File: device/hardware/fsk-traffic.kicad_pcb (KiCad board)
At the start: 2 copper layers, 79 x 41.5 mm, 43 parts, among them J1 JTAG, J2 USB_C, J3 2EDGV-5.08-03P, J4 2EDGV-5.08-03P, J5 2EDGV-5.08-03P, Q1 MMBT5551, Q2 AO3401A, Q3 MMBT5551, Q4 AO3401A, U1 XC6206P332MR, U2 MT3608, U3 STM32F070F6Px, Y1 12MHz

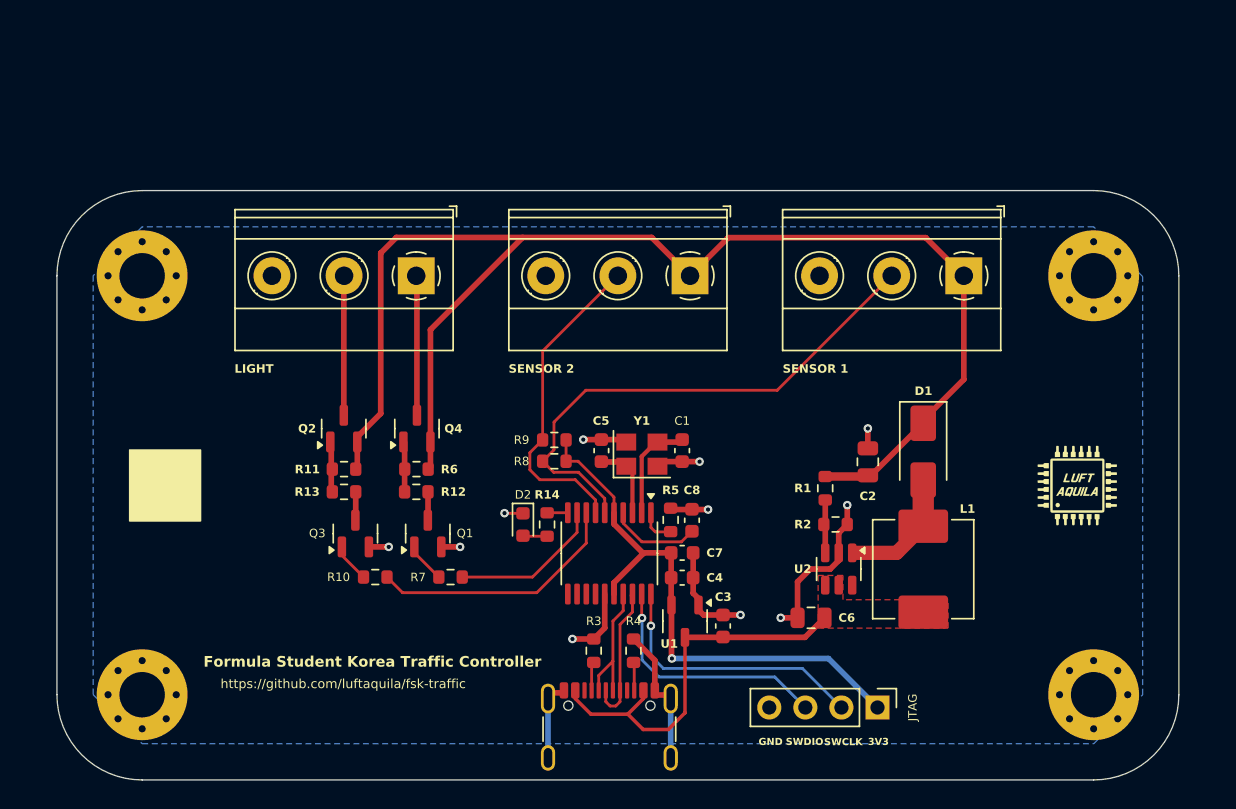
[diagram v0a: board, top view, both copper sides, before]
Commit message: fix: isolation & filter
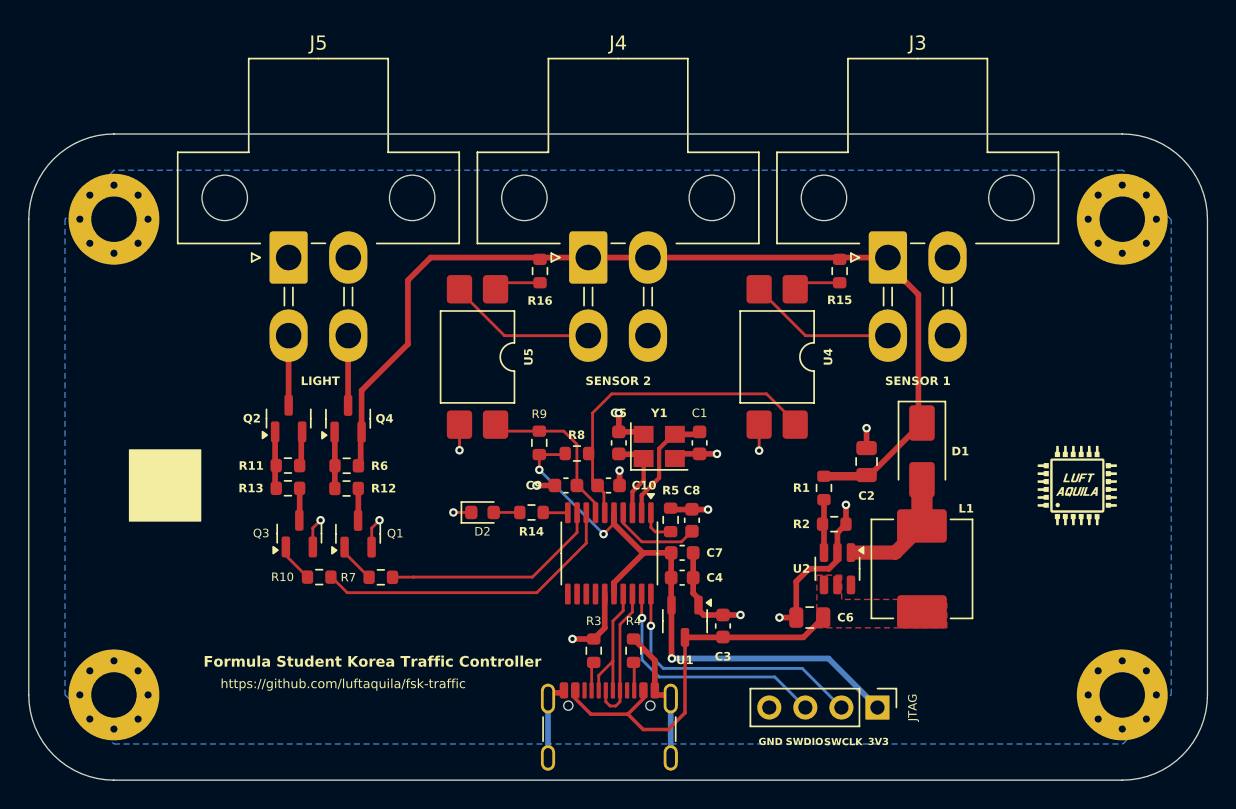
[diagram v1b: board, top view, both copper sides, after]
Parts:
- added C10: 470nF, Capacitor_SMD:C_0603_1608Metric, F.Cu at (143.5, 104.7)
- added C9: 470nF, Capacitor_SMD:C_0603_1608Metric, F.Cu at (140.5, 104.7)
- added R15: 2k, Resistor_SMD:R_0603_1608Metric, F.Cu at (159.8, 89.5)
- added R16: 2k, Resistor_SMD:R_0603_1608Metric, F.Cu at (138.7, 89.5)
- added U4: LTV-817S, Package_DIP:SMDIP-4_W9.53mm, F.Cu at (155.4, 95.6)
- added U5: LTV-817S, Package_DIP:SMDIP-4_W9.53mm, F.Cu at (134.3, 95.6)
- J3, J4, J5: value 2EDGV-5.08-03P -> Molex 5569-04A1; footprint TerminalBlock_Phoenix:TerminalBlock_Phoenix_MKDS-1,5-3-5.08_1x03_P5.08mm_Horizontal -> Connector_Molex:Molex_Mini-Fit_Jr_5569-04A1_2x02_P4.20mm_Horizontal
- R8, R9: value 1k -> 3.3k
- moved J5 9.08 mm to (121.0, 88.6), turned to 0 degrees
- moved J4 7.28 mm to (142.1, 88.6), turned to 0 degrees
- moved J3 5.50 mm to (163.2, 88.6), turned to 0 degrees
- moved R12 4.92 mm to (125.1, 104.9)
- moved R6 4.92 mm to (125.1, 103.3)
- moved Q1 4.91 mm to (125.9, 108.1)
- moved R7 4.91 mm to (127.5, 111.1)
- moved Q4 4.90 mm to (125.2, 100.0)
- moved REF** 4.47 mm to (179.7, 85.9)
- moved REF** 4.45 mm to (108.7, 85.9)
- moved R11 3.96 mm to (121.0, 103.2)
- moved R13 3.96 mm to (121.0, 104.8)
- moved Q2 3.95 mm to (121.0, 99.9)
- moved Q3 3.95 mm to (121.8, 108.0)
- moved R10 3.95 mm to (123.2, 111.1)
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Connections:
- J3 pad 2: SENS1 -> unconnected-(J3-Pin_2-Pad2)
- J3 pad 3: GND -> Net-(J3-Pin_3)
- J4 pad 2: SENS2 -> 18V
- J4 pad 3: GND -> Net-(J4-Pin_3)
- J5 pad 1: /GN -> GND
- J5 pad 2: /RD -> unconnected-(J5-Pin_2-Pad2)
- J5 pad 3: GND -> /RD
- R8 pad 1: +3V3 -> SENS1
- R8 pad 2: SENS1 -> +3V3
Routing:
- net 18V: track 99.9 -> 73.1 mm
- net SENS1: track 37.6 -> 23.7 mm
- net SENS2: track 22.6 -> 11.7 mm
- net Net-(J4-Pin_3): track 0.00 -> 10.5 mm
- net Net-(J3-Pin_3): track 0.00 -> 10.4 mm
- net GND: track 52.8 -> 60.3 mm, vias 11 -> 15
- net GREEN: track 10.8 -> 15.7 mm
- net /GN: track 9.85 -> 5.01 mm
- net /RD: track 9.83 -> 5.01 mm
- net Net-(R16-Pad2): track 0.00 -> 4.09 mm
- net RED: track 18.1 -> 22.0 mm
- net +3V3: track 40.5 -> 44.3 mm, vias 1 -> 3
- net Net-(R15-Pad2): track 0.00 -> 3.34 mm
- net OSC_IN: track 7.16 -> 8.21 mm
- net OSC_OUT: track 5.04 -> 5.73 mm
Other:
- board size 79 x 41.5 mm -> 83 x 45.5 mm
